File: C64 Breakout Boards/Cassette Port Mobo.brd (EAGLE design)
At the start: 60.4 x 31.2 mm, 2 parts

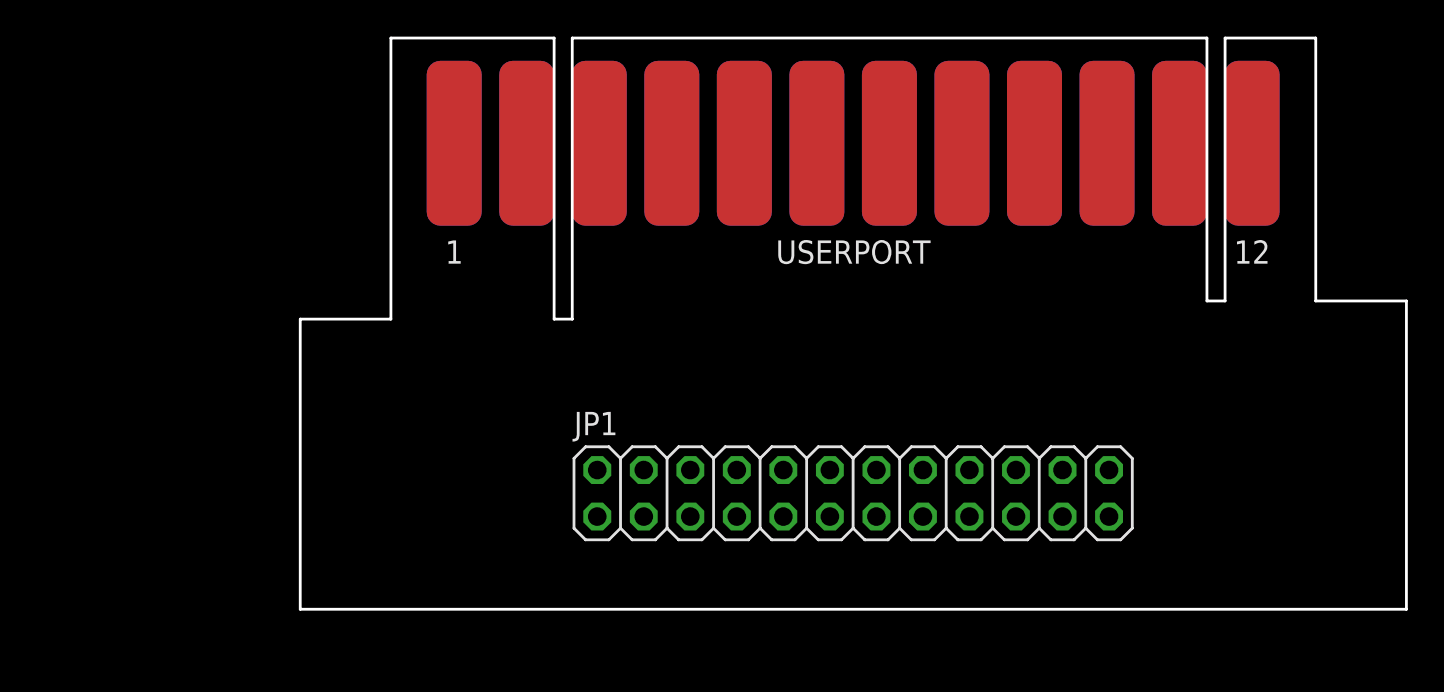
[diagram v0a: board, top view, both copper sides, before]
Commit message: More expansion board work
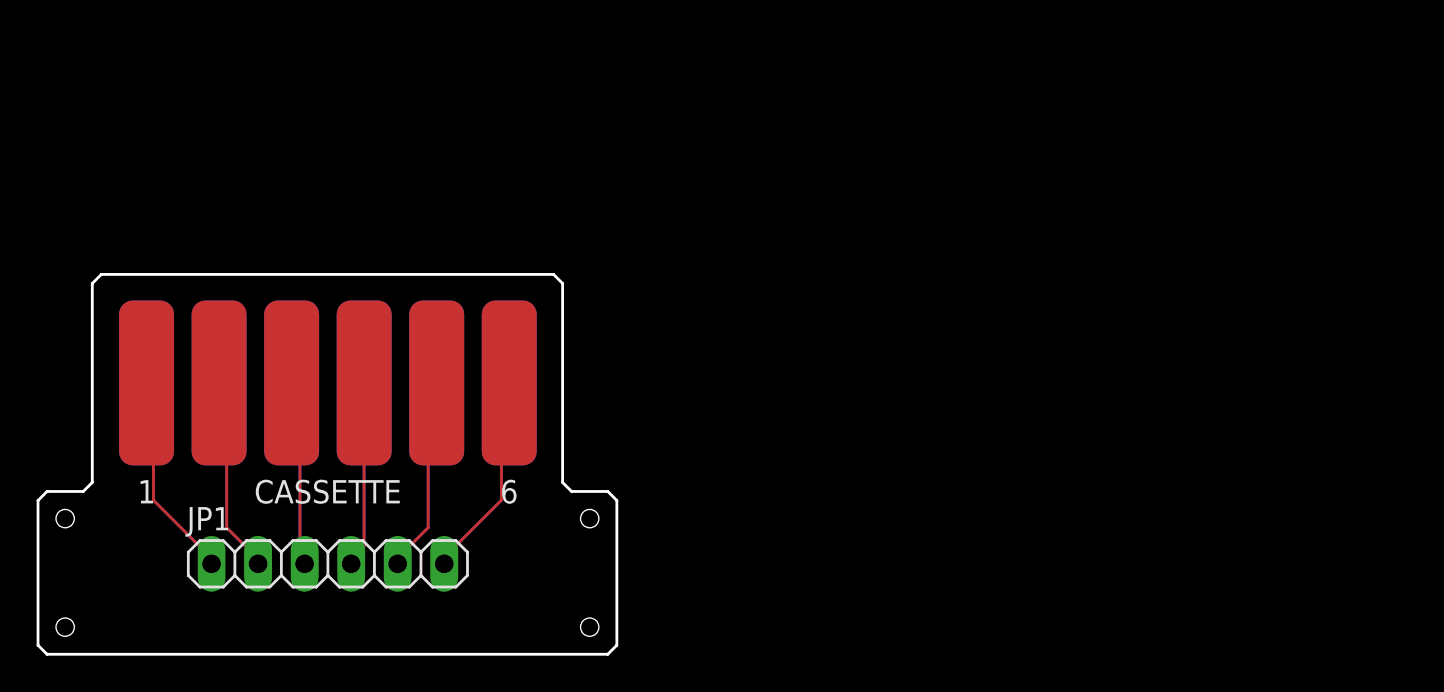
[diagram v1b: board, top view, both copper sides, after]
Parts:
- removed USERPORT: C64_USER, 0myparts:C64_USER
- added CASSETTE: C64_CASSETTE, 0myparts:C64_CASSETTE
- JP1: device pinhead:2X12 -> pinhead:1X06
- moved JP1 28.9 mm to (0.03, -1.98)
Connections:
- removed net !FLAG2: JP1.14, USERPORT.!FLAG2
- removed net !PC2: JP1.8, USERPORT.!PC2
- removed net !RESET: JP1.3, USERPORT.!RESET
- removed net 9VAC+: JP1.10, USERPORT.9VAC+
- removed net 9VAC-: JP1.11, USERPORT.9VAC-
- removed net ATN: JP1.9, USERPORT.ATN
- removed net CNT1: JP1.4, USERPORT.CNT1
- removed net CNT2: JP1.6, USERPORT.CNT2
- removed net GND: JP1.1, JP1.12, JP1.13, JP1.24, USERPORT.GND1, USERPORT.GND2, USERPORT.GND3, USERPORT.GND4
- removed net PA2: JP1.23, USERPORT.PA2
- removed net PB0: JP1.15, USERPORT.PB0
- removed net PB1: JP1.16, USERPORT.PB1
- removed net PB2: JP1.17, USERPORT.PB2
- removed net PB3: JP1.18, USERPORT.PB3
- removed net PB4: JP1.19, USERPORT.PB4
- removed net PB5: JP1.20, USERPORT.PB5
- removed net PB6: JP1.21, USERPORT.PB6
- removed net PB7: JP1.22, USERPORT.PB7
- removed net SP1: JP1.5, USERPORT.SP1
- removed net SP2: JP1.7, USERPORT.SP2
- removed net VCC: JP1.2, USERPORT.VCC
- new net GND1: CASSETTE.GND1, CASSETTE.GND2, JP1.1
- new net MOTOR1: CASSETTE.MOTOR1, CASSETTE.MOTOR2, JP1.3
- new net READ1: CASSETTE.READ1, CASSETTE.READ2, JP1.4
- new net SENSE1: CASSETTE.SENSE1, CASSETTE.SENSE2, JP1.6
- new net VCC1: CASSETTE.VCC1, CASSETTE.VCC2, JP1.2
- new net WRITE1: CASSETTE.WRITE1, CASSETTE.WRITE2, JP1.5
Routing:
- net SENSE1: track 0.00 -> 22.6 mm
- net GND1: track 0.00 -> 22.6 mm
- net WRITE1: track 0.00 -> 21.5 mm
- net VCC1: track 0.00 -> 21.4 mm
- net MOTOR1: track 0.00 -> 20.3 mm
- net READ1: track 0.00 -> 20.2 mm
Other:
- board size 60.4 x 31.2 mm -> 31.6 x 20.7 mm
